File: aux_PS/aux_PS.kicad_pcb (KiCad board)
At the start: 2 copper layers, 92.2 x 69 mm, 15 parts, among them J1 P78E03-1000, J2 Conn_02x03_Counter_Clockwise

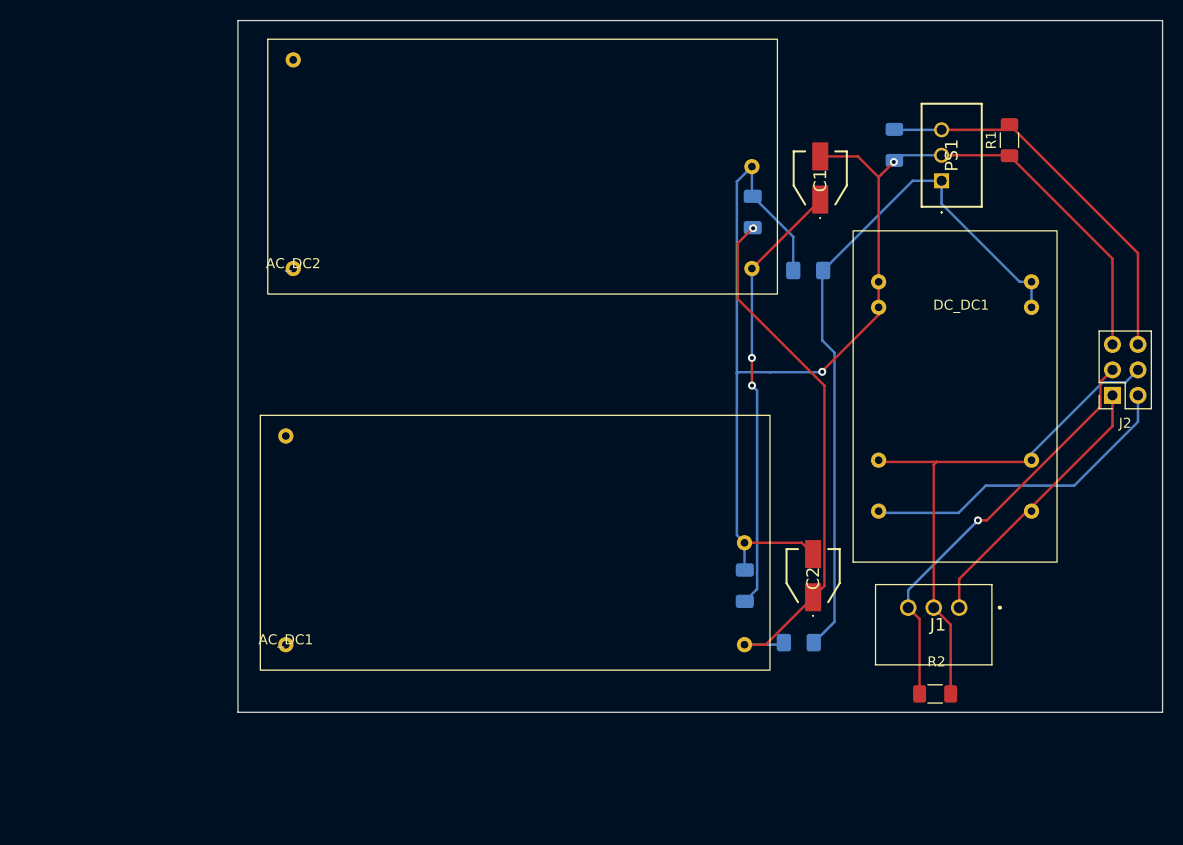
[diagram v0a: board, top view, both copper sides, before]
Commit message: header design
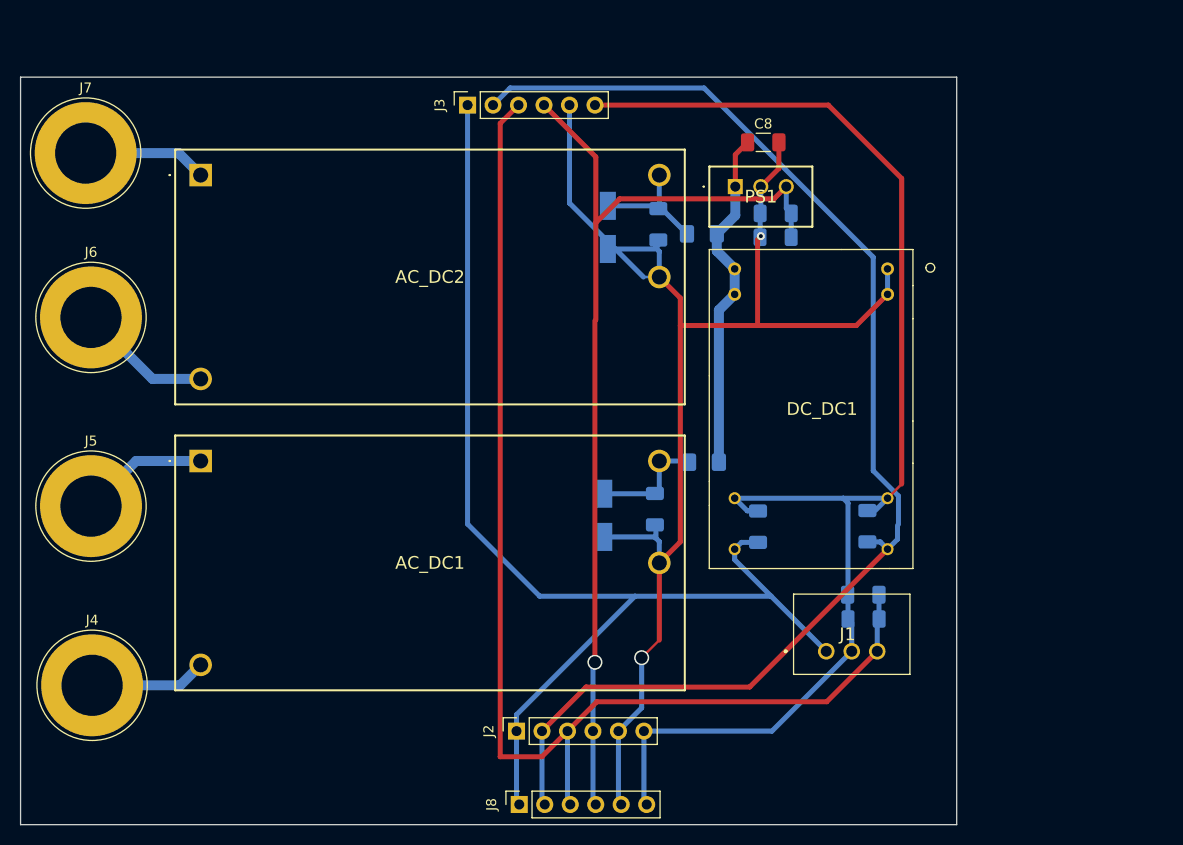
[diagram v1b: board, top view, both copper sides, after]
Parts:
- added C6: 1u_cer, Capacitor_SMD:C_1206_3216Metric_Pad1.33x1.80mm_HandSolder, B.Cu at (118.8, 94.0)
- added C7: 1u_cer, Capacitor_SMD:C_1206_3216Metric_Pad1.33x1.80mm_HandSolder, B.Cu at (129.7, 94.0)
- added C8: 1u_cer, Capacitor_SMD:C_1206_3216Metric_Pad1.33x1.80mm_HandSolder, F.Cu at (119.3, 55.7)
- added C9: 1u_cer, Capacitor_SMD:C_1206_3216Metric_Pad1.33x1.80mm_HandSolder, B.Cu at (129.3, 100.8)
- added J3: Conn_01x06, Connector_PinSocket_2.54mm:PinSocket_1x06_P2.54mm_Vertical, F.Cu at (89.9, 52.0)
- added J4: Conn_01x01_Female, Connector:Banana_Jack_1Pin, F.Cu at (52.5, 109.8)
- added J5: Conn_01x01_Female, Connector:Banana_Jack_1Pin, F.Cu at (52.3, 92.0)
- added J6: Conn_01x01_Female, Connector:Banana_Jack_1Pin, F.Cu at (52.3, 73.2)
- added J7: Conn_01x01_Female, Connector:Banana_Jack_1Pin, F.Cu at (51.8, 56.8)
- added J8: Conn_01x06, Connector_PinSocket_2.54mm:PinSocket_1x06_P2.54mm_Vertical, F.Cu at (95.0, 121.7)
- AC_DC1, AC_DC2: footprint PSK-S6C-24:PSK-S6C-24 -> PSK-S6C-24:PSKS6C24
- C1, C2, R1, R2: moved to B.Cu
- DC_DC1: footprint DCWN-06B:DCWN-06B -> DCWN-06B:DCWN06B15
- J2: value Conn_02x03_Counter_Clockwise -> Conn_01x06; footprint Connector_PinSocket_2.54mm:PinSocket_2x03_P2.54mm_Vertical -> Connector_PinSocket_2.54mm:PinSocket_1x06_P2.54mm_Vertical
- moved J2 68.2 mm to (94.8, 114.4), turned to 90 degrees
- moved C3 37.0 mm to (108.9, 63.9), turned to -90 degrees
- moved C4 31.2 mm to (108.6, 92.3), turned to -90 degrees
- moved DC_DC1 25.4 mm to (124.1, 82.3)
- moved R1 24.4 mm to (120.6, 62.8), turned to 0 degrees
- moved C1 21.7 mm to (103.9, 64.2), turned to -90 degrees
- moved C2 21.7 mm to (103.5, 92.9), turned to -90 degrees
- moved PS1 20.6 mm to (116.6, 60.1), turned to 0 degrees
- moved D1 20.3 mm to (113.4, 87.6)
- moved AC_DC1 20.2 mm to (63.3, 87.5)
- moved C5 15.0 mm to (120.6, 65.2), turned to 0 degrees
- moved J1 13.9 mm to (125.6, 106.4), turned to 0 degrees
- moved AC_DC2 13.1 mm to (63.3, 59.0)
- moved D2 11.2 mm to (113.2, 64.8)
- moved R2 10.3 mm to (129.3, 103.2), turned to 0 degrees
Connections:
- AC_DC1 pad 1: unconnected-(AC_DC1-Pad1) -> Net-(AC_DC1-Pad1)
- AC_DC1 pad 2: unconnected-(AC_DC1-Pad2) -> Net-(AC_DC1-Pad2)
- AC_DC2 pad 1: unconnected-(AC_DC2-Pad1) -> Net-(AC_DC2-Pad1)
- AC_DC2 pad 2: unconnected-(AC_DC2-Pad2) -> Net-(AC_DC2-Pad2)
- D2 pad 1: 24_gnd -> Net-(AC_DC2-Pad4)
- J2 pad 4: ctrl_gnd -> V12
- J2 pad 6: V12 -> ctrl_gnd
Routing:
- net ctrl_-15: track 32.9 -> 127.9 mm
- net ctrl_15: track 27.5 -> 117.3 mm
- net ctrl_gnd: track 53.9 -> 133.8 mm
- net ctrl_3v3: track 41.7 -> 120.8 mm, vias 1 -> 0
- net V12: track 38.9 -> 107.5 mm, vias 0 -> 1
- net Net-(AC_DC1-Pad4): track 54.3 -> 11.5 mm, vias 1 -> 0
- net /V_24: track 71.0 -> 34.5 mm
- net Net-(AC_DC2-Pad4): track 43.6 -> 12.4 mm, vias 2 -> 0
- net Net-(AC_DC2-Pad2): track 0.00 -> 13.5 mm
- net Net-(AC_DC1-Pad1): track 0.00 -> 12.8 mm
- net Net-(AC_DC2-Pad1): track 0.00 -> 12.4 mm
- net Net-(AC_DC1-Pad2): track 0.00 -> 11.7 mm
- net 24_gnd: track 134.6 -> 140.2 mm
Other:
- board size 92.2 x 69 mm -> 93.3 x 74.5 mm
